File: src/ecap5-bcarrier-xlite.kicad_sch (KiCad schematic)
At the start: 43 parts, among them J3 Conn_01x04, J4 Conn_01x04, J5 USB_C_Receptacle_USB2.0_14P, J6 Conn_Coaxial, J7 Conn_Coaxial, J8 Conn_Coaxial, J9 1935161, Q1 BC846BR13, Q2 BC846BR13, SW1 RESET_SOM1, SW2 RESET_SOM2, SW3 USER1, SW4 USER1, U2 AP7375-33SA-7

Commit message: Save button footprint in local library
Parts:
- SW1, SW2, SW3, SW4: footprint Button_Switch_SMD:SW_Push_1P1T_NO_CK_PTS125Sx73SMTR -> ECAP5-BCARRIER-XLITE:SW_Push_1P1T_NO_CK_PTS125Sx73SMTR_1
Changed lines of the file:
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@@
 			)
 		)
-		(property "Footprint" "Button_Switch_SMD:SW_Push_1P1T_NO_CK_PTS125Sx73SMTR"
+		(property "Footprint" "ECAP5-BCARRIER-XLITE:SW_Push_1P1T_NO_CK_PTS125Sx73SMTR_1"
 			(at 107.95 125.73 0)
 			(effects
@@
 			)
 		)
-		(property "Footprint" "Button_Switch_SMD:SW_Push_1P1T_NO_CK_PTS125Sx73SMTR"
+		(property "Footprint" "ECAP5-BCARRIER-XLITE:SW_Push_1P1T_NO_CK_PTS125Sx73SMTR_1"
 			(at 72.39 125.73 0)
 			(effects
@@
 			)
 		)
-		(property "Footprint" "Button_Switch_SMD:SW_Push_1P1T_NO_CK_PTS125Sx73SMTR"
+		(property "Footprint" "ECAP5-BCARRIER-XLITE:SW_Push_1P1T_NO_CK_PTS125Sx73SMTR_1"
 			(at 109.22 147.32 0)
 			(effects
@@
 			)
 		)
-		(property "Footprint" "Button_Switch_SMD:SW_Push_1P1T_NO_CK_PTS125Sx73SMTR"
+		(property "Footprint" "ECAP5-BCARRIER-XLITE:SW_Push_1P1T_NO_CK_PTS125Sx73SMTR_1"
 			(at 73.66 147.32 0)
 			(effects

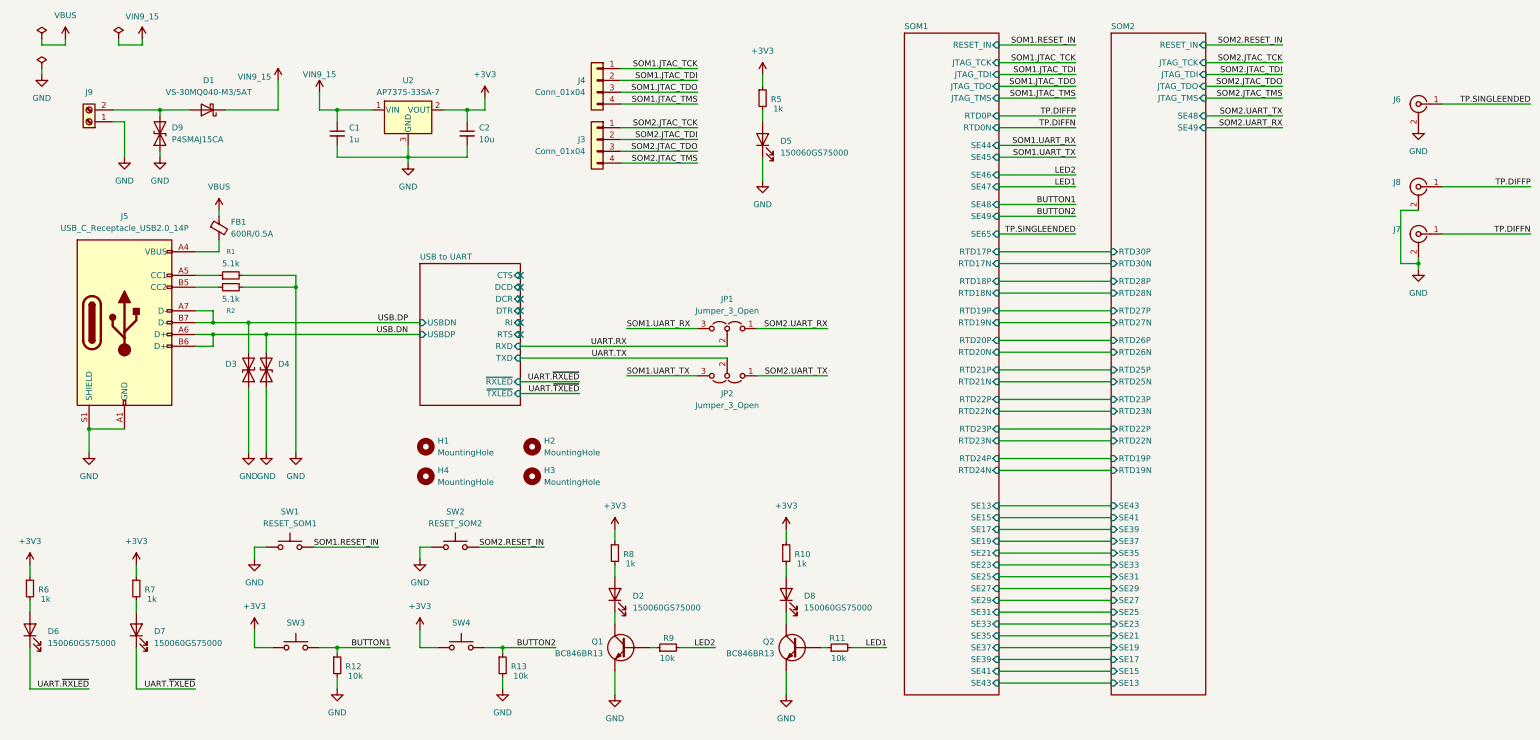
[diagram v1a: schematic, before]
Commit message: Improve the schematic
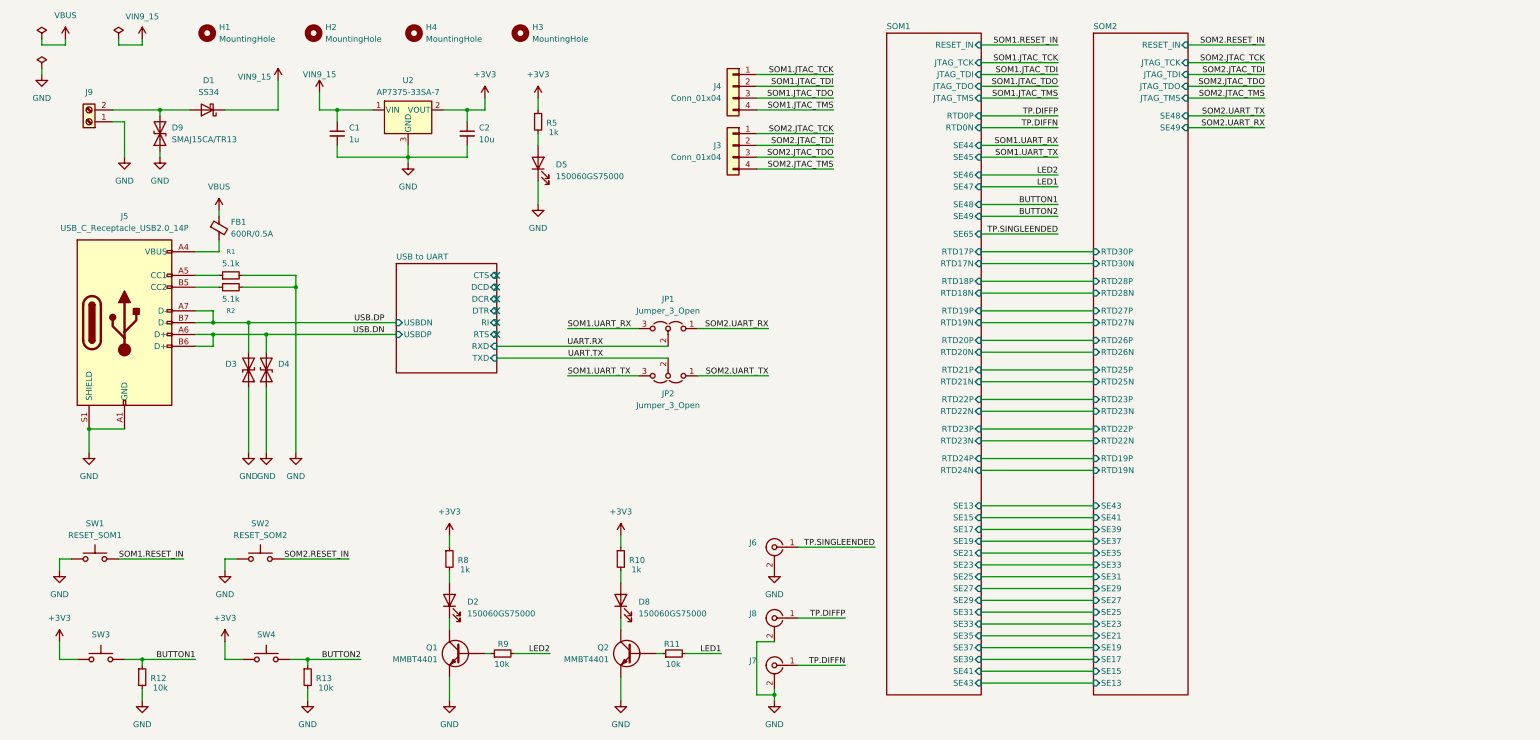
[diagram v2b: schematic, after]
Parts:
- removed D6, D7: 150060GS75000, LED_SMD:LED_0603_1608Metric, symbol Device:LED
- removed R6, R7: 1k, Resistor_SMD:R_0603_1608Metric, symbol Device:R_Small
- C1: MPN (none) -> CL10A105KB8NNNC
- C2: MPN (none) -> CL10A106KP8NNNC
- D1: value VS-30MQ040-M3/5AT -> SS34; MPN (none) -> SS34
- D2, D5, D8: MPN (none) -> 150060GS75000
- D3, D4: MPN (none) -> ESD321DYAR
- D9: value P4SMAJ15CA -> SMAJ15CA/TR13; MPN (none) -> SMAJ15CA/TR13
- FB1: MPN (none) -> GZ2012D601TF
- J5: MPN (none) -> USB4105-GF-A-060
- J6, J7, J8: MPN (none) -> 132134-10
- J9: value 1935161 -> WJ127-5.0-2P; MPN (none) -> WJ127-5.0-2P
- JP1, JP2: now in the parts list
- Q1, Q2: value BC846BR13 -> MMBT4401; MPN (none) -> MMBT4401
- R1, R2: MPN (none) -> 0603WAF5101T5E
- R10, R5, R8: MPN (none) -> 0603WAF1001T5E
- R11, R12, R13, R9: MPN (none) -> 0603WAF1002T5E
- SW1, SW2, SW3, SW4: footprint ECAP5-BCARRIER-XLITE:SW_Push_1P1T_NO_CK_PTS125Sx73SMTR_1 -> Button_Switch_SMD:SW_Push_1P1T_NO_CK_PTS125Sx43PSMTR
- U2: MPN (none) -> AP7375-33SA-7
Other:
- sheet USB to UART ports: added none; removed ~{RXLED}, ~{TXLED}
- title: (none) -> ECAP5-BCARRIER-XLITE
- moved on the sheet: D2, D5, D8, H1, H2, H3, H4, J3, J4, J6, J7, J8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
